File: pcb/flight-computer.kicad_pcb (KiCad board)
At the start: 4 copper layers, 83.7 x 62.9 mm, 83 parts, among them J1 MicroSD Slot, J2 USB_C_Receptacle_USB2.0_16P, J3 SMA_Coax, J4 Conn_01x02, J5 ARM, Q1 PMOS, SW1 SW_Push, SW2 SW_Push, U1 RP2040, U10 LM3671MF, U11 TPS2116DRL, U2 W25Q16JVSS, U3 USBLC6-2SC6, U4 M24C32-FMN, U5 MS5607-02BA, U6 LIS2MDL, U7 LSM6DSO32TR, U8 LC86G, U9 RN2903, Y1 12MHz

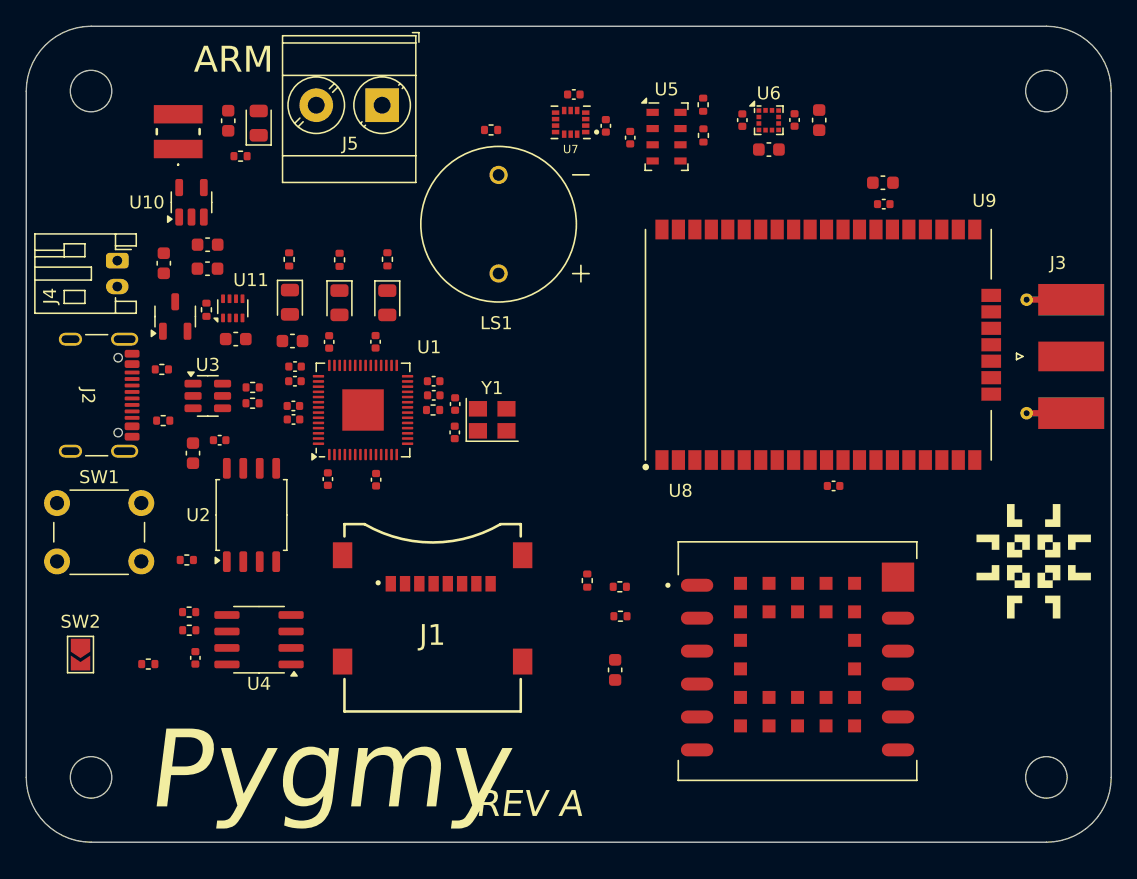
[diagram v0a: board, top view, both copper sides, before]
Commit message: Almost done routing
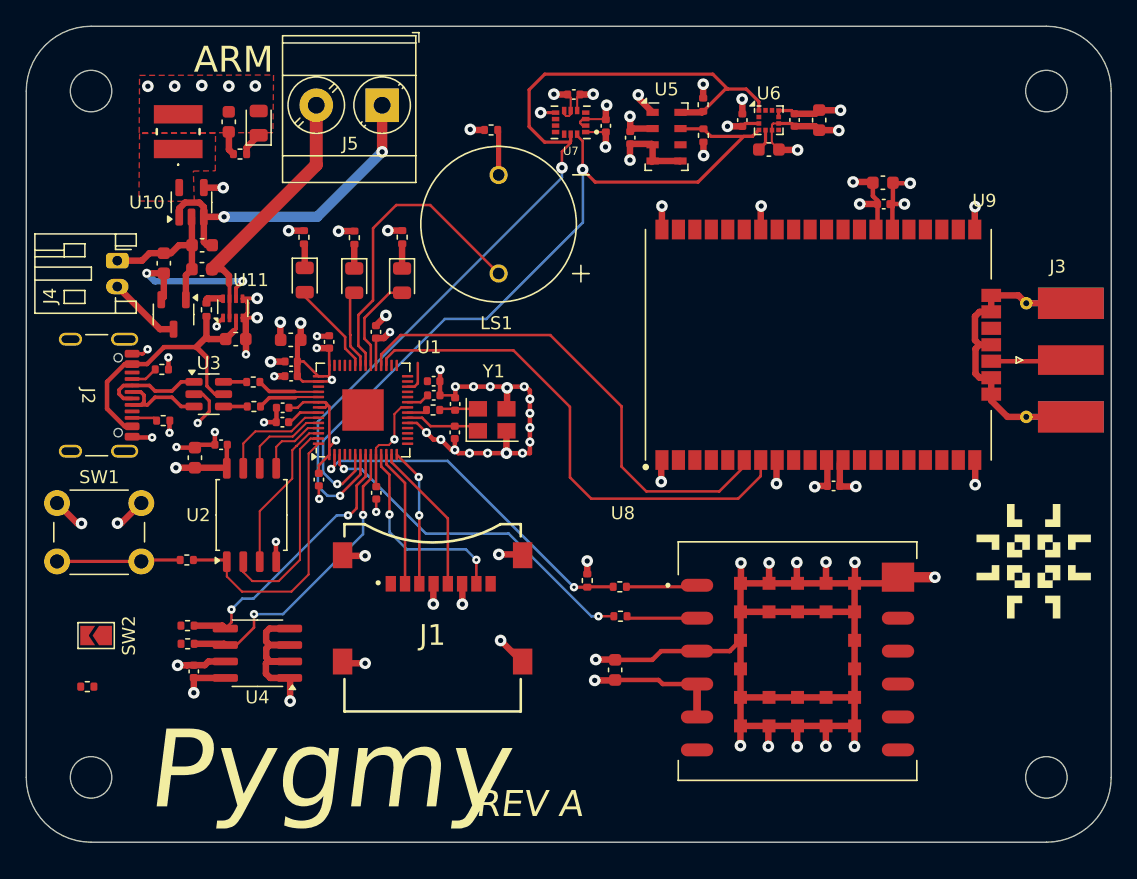
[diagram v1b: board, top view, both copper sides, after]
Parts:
- moved R1 5.02 mm to (88.9, 121.5)
- moved D1 2.06 mm to (105.7, 90.2)
- moved D3 2.06 mm to (113.2, 90.2)
- moved R12 2.06 mm to (105.6, 86.9)
- moved R13 2.06 mm to (109.5, 86.9)
- moved D2 2.06 mm to (109.5, 90.2)
- moved R14 2.06 mm to (113.2, 86.9)
- moved SW2 1.90 mm to (89.6, 117.6), turned to 180 degrees
- moved C19 1.05 mm to (97.1, 120.4)
- moved R6 1.05 mm to (96.6, 118.2)
- moved U4 1.05 mm to (102.0, 119.0)
- moved R5 1.05 mm to (96.6, 116.8)
- moved C11 1.01 mm to (111.2, 106.6)
- moved C6 0.88 mm to (104.0, 101.1)
- moved C13 0.84 mm to (104.0, 100.0)
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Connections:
- net Net-(U1-USB_DM) renamed /RD-
- net Net-(U1-USB_DP) renamed /RD+
- net Net-(U10-SW) renamed /Power/NSY_OUT
- Q1 pad 1: /Power/BAT+ -> GND
- Q1 pad 2: GND -> +3V7
- Q1 pad 3: +3V7 -> /Power/BAT+
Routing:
- net GND: track 0.00 -> 268.0 mm, vias 0 -> 78
- net +3V3: track 0.00 -> 90.1 mm, vias 0 -> 28
- net I2C0_SCL: track 0.00 -> 72.4 mm, vias 0 -> 2
- net I2C0_SDA: track 0.00 -> 62.4 mm, vias 0 -> 2
- net MCU_UART1_TX: track 0.00 -> 39.6 mm
- net MCU_UART1_RX: track 0.00 -> 38.5 mm
- net MCU_UART0_TX: track 0.00 -> 27.3 mm, vias 0 -> 2
- net MCU_UART0_RX: track 0.00 -> 26.8 mm, vias 0 -> 2
- net /Power/REGULATOR_IN: track 0.00 -> 25.8 mm, vias 0 -> 2
- net I2C1_SCL: track 0.00 -> 24.3 mm, vias 0 -> 2
- net /BUZZ: track 0.00 -> 23.9 mm
- net +5V: track 0.00 -> 23.7 mm
- net /QSPI_SS: track 0.00 -> 21.5 mm
- net I2C1_SDA: track 0.00 -> 21.5 mm, vias 0 -> 2
- net /Power/PWR_SRC: track 0.00 -> 20.8 mm
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- added copper zone on F.Cu, net +3V3
- added copper zone on F.Cu, net /Power/NSY_OUT
